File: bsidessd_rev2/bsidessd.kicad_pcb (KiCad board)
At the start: 2 copper layers, 50 x 50 mm, 26 parts, among them J1 Conn_01x05, J2 Conn_01x05, J3 USB_B_Micro, SW1 PTS810, U1 ATSAMD21E18A-AUT, U2 AP2112K-3.3

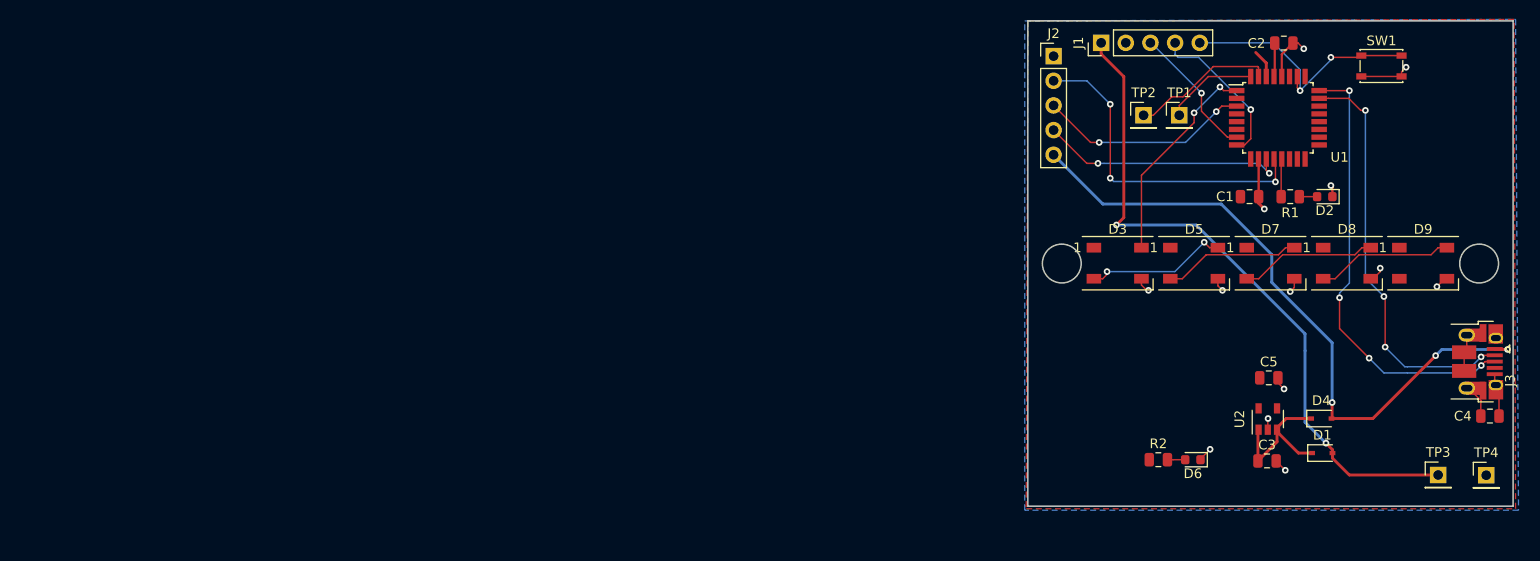
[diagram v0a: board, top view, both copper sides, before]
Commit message: Passes DRC :) Need a sanity check before ordering.
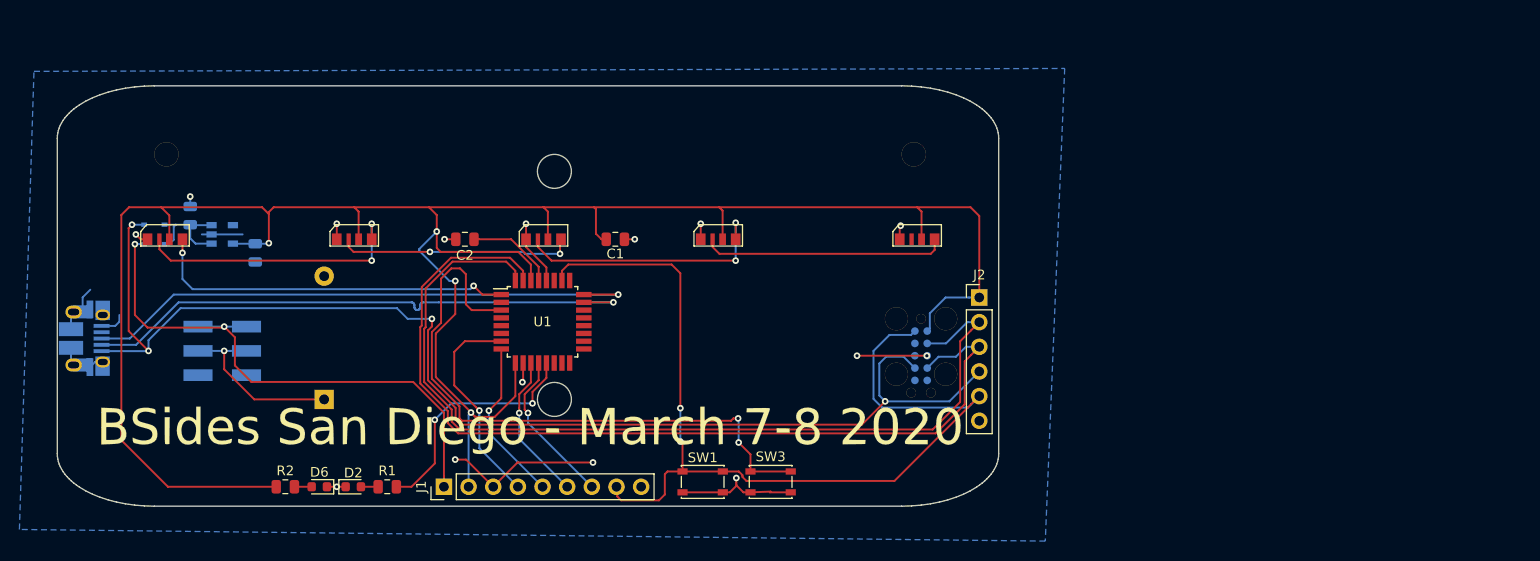
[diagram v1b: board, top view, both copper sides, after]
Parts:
- removed C4: 1nF, Capacitor_SMD:C_0805_2012Metric
- removed D3, D5, D7, D8, D9: WS2812B, LED_SMD:LED_WS2812B_PLCC4_5.0x5.0mm_P3.2mm
- removed TP1: SWD, Connector_PinHeader_2.54mm:PinHeader_1x01_P2.54mm_Vertical
- removed TP2: SWC, Connector_PinHeader_2.54mm:PinHeader_1x01_P2.54mm_Vertical
- removed TP3: Battery, Connector_PinHeader_2.54mm:PinHeader_1x01_P2.54mm_Vertical
- removed TP4: Ground, Connector_PinHeader_2.54mm:PinHeader_1x01_P2.54mm_Vertical
- added BT1: 3xAAA Keystone 2479, Battery:BatteryHolder_Keystone_2479_3xAAA, B.Cu at (77.5, 139.0)
- added SW2: JS202011SCQN, andnxor:JS202011SCQN, B.Cu at (67.0, 134.0)
- added SW3: USER Button, Button_Switch_SMD:SW_SPST_PTS810, F.Cu at (123.5, 147.5)
- added TC1: Tag Connect 2050, andnxor:TC2050-IDC-FP-NoSilk, B.Cu at (139.0, 134.5)
- added U3: sk6812_side, andnxor:LED_SK6812_SIDE, F.Cu at (61.0, 122.5)
- added U4: sk6812_side, andnxor:LED_SK6812_SIDE, F.Cu at (80.5, 122.5)
- added U5: sk6812_side, andnxor:LED_SK6812_SIDE, F.Cu at (100.0, 122.5)
- added U6: sk6812_side, andnxor:LED_SK6812_SIDE, F.Cu at (118.0, 122.5)
- added U7: sk6812_side, andnxor:LED_SK6812_SIDE, F.Cu at (138.5, 122.5)
- added g1: graphic, bsidessd_rev2:bsidessd_rev2, F.Cu at (100.0, 100.0)
- C3, C5, D1, D4, J3, U2: moved to B.Cu
- J1: value Conn_01x05 -> Conn_01x09; footprint Connector_PinHeader_2.54mm:PinHeader_1x05_P2.54mm_Vertical -> Connector_PinHeader_2.54mm:PinHeader_1x09_P2.54mm_Vertical
- J2: value Conn_01x05 -> SWD; footprint Connector_PinHeader_2.54mm:PinHeader_1x05_P2.54mm_Vertical -> Connector_PinHeader_2.54mm:PinHeader_1x06_P2.54mm_Vertical
- SW1: value PTS810 -> RESET Button
- moved J3 143.6 mm to (52.8, 132.7), turned to 90 degrees
- moved D1 122.3 mm to (60.0, 123.0), turned to 180 degrees
- moved D4 121.9 mm to (60.0, 121.0), turned to 180 degrees
- moved C3 113.8 mm to (63.7, 120.1), turned to 90 degrees
- moved U2 109.4 mm to (67.0, 122.0), turned to 0 degrees
- moved C5 105.2 mm to (70.4, 123.9), turned to 270 degrees
- moved D2 104.5 mm to (80.5, 148.0), turned to 0 degrees
- moved R1 97.7 mm to (84.0, 148.0), turned to 0 degrees
- moved D6 90.0 mm to (77.0, 148.0)
- moved R2 90.0 mm to (73.5, 148.0)
- moved C2 86.8 mm to (92.0, 122.5), turned to 180 degrees
- moved SW1 82.0 mm to (116.5, 147.5), turned to 180 degrees
- moved J1 81.7 mm to (89.8, 148.0)
- moved U1 78.6 mm to (100.0, 131.0)
- moved C1 65.5 mm to (107.5, 122.5)
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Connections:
- net /D+ renamed USB_DP
- net /D- renamed USB_DM
- J1 pad 2: GND -> +3V3
- J1 pad 3: /D4_A2_PAU06_TXD_MOSI -> GND
- J1 pad 4: /D3_A3_PAU07_RXD_SCK -> /D4_A2_PAU06_TXD_MOSI
- J1 pad 5: /~RESET -> /D3_A3_PAU07_RXD_SCK
- J2 pad 2: /D2_A1_PAU09_SCL_MISO -> SWDIO
- J2 pad 3: /D1_A0_PAU02 -> SWCLK
- J2 pad 4: /D0_A4_PAU08_SDA -> VBUS
- J2 pad 5: VBUS -> /~RESET
- SW1 pad 1: /~RESET -> GND
- SW1 pad 2: GND -> /~RESET
- U1 pad 1: /LED -> LED
- U1 pad 31: Net-(TP2-Pad1) -> SWCLK
- U1 pad 32: Net-(TP1-Pad1) -> SWDIO
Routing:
- net +3V3: track 2.93 -> 232.5 mm, vias 0 -> 4
- net SWCLK: track 0.00 -> 96.3 mm
- net SWDIO: track 0.00 -> 95.9 mm
- net /~RESET: track 27.3 -> 101.7 mm
- net VBUS: track 68.7 -> 129.0 mm, vias 3 -> 4
- net /D1_A0_PAU02: track 22.0 -> 65.3 mm
- net LED: track 0.00 -> 37.9 mm, vias 0 -> 2
- net GND: track 42.0 -> 71.1 mm, vias 13 -> 15
- net Net-(U3-Pad3): track 0.00 -> 28.8 mm, vias 0 -> 2
- net Net-(U5-Pad3): track 0.00 -> 27.4 mm, vias 0 -> 2
- net Net-(U6-Pad3): track 0.00 -> 25.2 mm
- net Net-(U4-Pad3): track 0.00 -> 24.4 mm, vias 0 -> 2
- net /LED: track 21.8 -> 0.00 mm, vias 2 -> 0
- net Net-(R1-Pad2): track 3.91 -> 25.0 mm, vias 0 -> 2
- net Net-(BT1-Pad1): track 0.00 -> 18.5 mm, vias 0 -> 1
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- removed copper zone on F.Cu, net +3V3
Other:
- board size 50 x 50 mm -> 97 x 43.3 mm
- net class Default: clearance 0.1524 -> 0.2; trace_width 0.1524 -> 0.2
- rule trace_clearance: 0.1524 -> 0.2
